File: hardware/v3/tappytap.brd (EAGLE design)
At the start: 36 x 16 mm, 18 parts

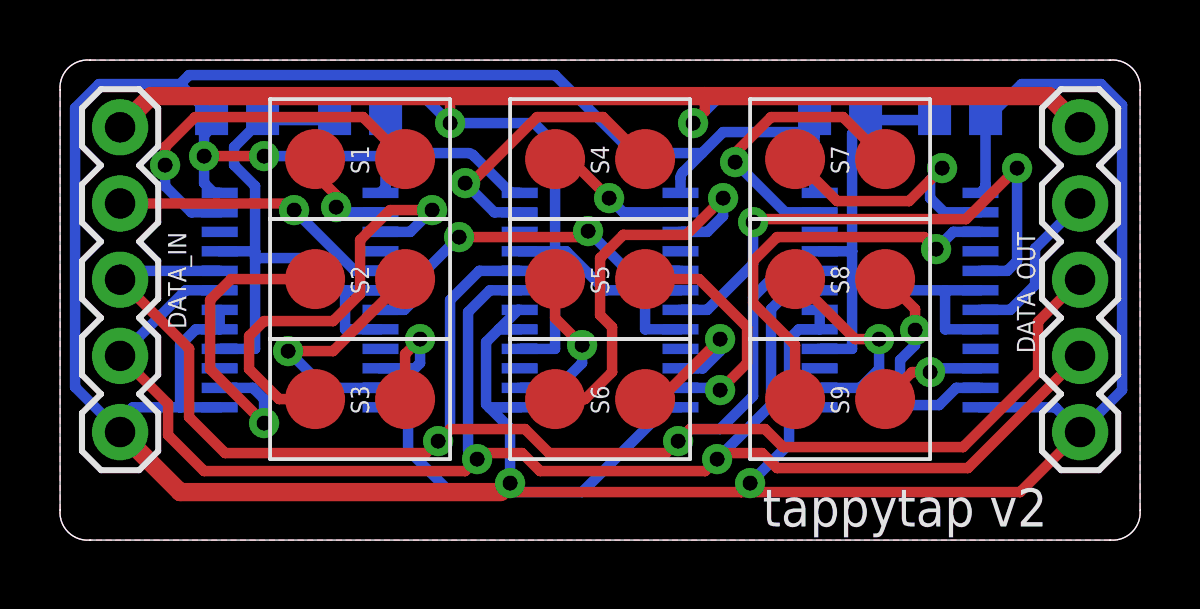
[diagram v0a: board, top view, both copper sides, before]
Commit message: Tappytap v3 design done with gerbers
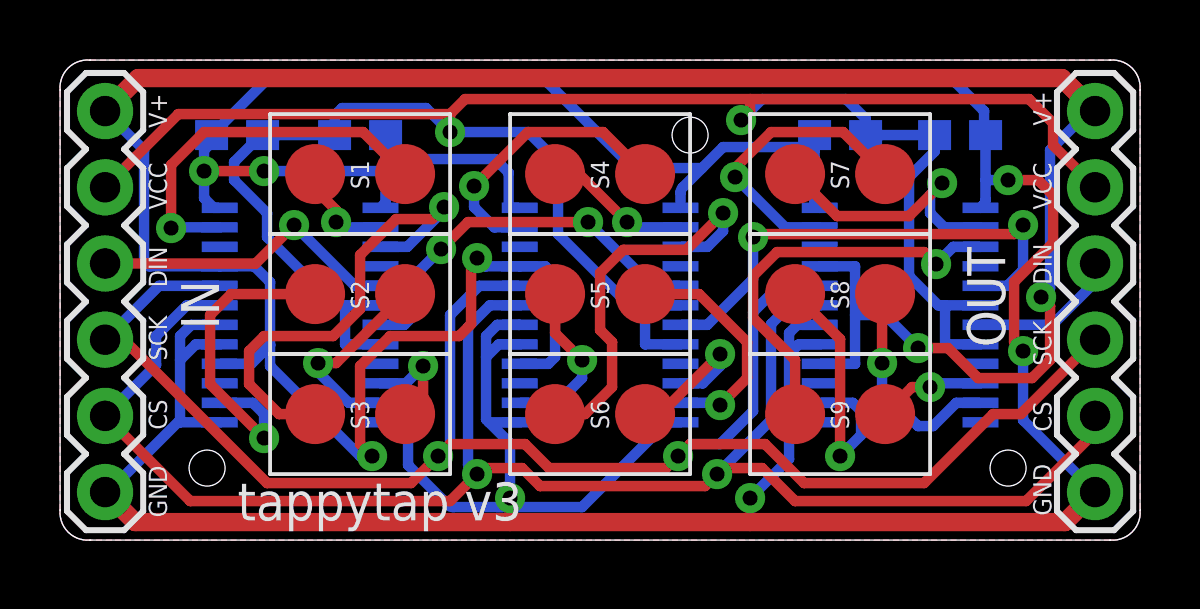
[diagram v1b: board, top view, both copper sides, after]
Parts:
- removed DATA_IN, DATA_OUT: (no value), SparkFun-Connectors:1X05
- added IN, OUT: (no value), SparkFun-Connectors:1X06
- moved C1 0.50 mm to (5.90, 12.5)
- moved C2 0.50 mm to (10.0, 12.5)
- moved C3 0.50 mm to (26.0, 12.5)
- moved C4 0.50 mm to (30.0, 12.5)
- moved HBR1 0.50 mm to (8.00, 6.50)
- moved HBR2 0.50 mm to (18.0, 6.50)
- moved HBR3 0.50 mm to (28.0, 6.50)
- moved S1 0.50 mm to (10.0, 11.2)
- moved S2 0.50 mm to (10.0, 7.20)
- moved S3 0.50 mm to (10.0, 3.20)
- moved S4 0.50 mm to (18.0, 11.2)
- moved S5 0.50 mm to (18.0, 7.20)
- moved S6 0.50 mm to (18.0, 3.20)
- moved S7 0.50 mm to (26.0, 11.2)
- moved S8 0.50 mm to (26.0, 7.20)
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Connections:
- new net V+: HBR1.16, HBR1.21, HBR2.16, HBR2.21, HBR3.16, HBR3.21, IN.6, OUT.6
- net +5V: now also IN.5, OUT.5; no longer DATA_IN.5, DATA_OUT.5, HBR1.16, HBR1.21, HBR2.16, HBR2.21, HBR3.16, HBR3.21
- net GND: now also IN.1, OUT.1; no longer DATA_IN.1, DATA_OUT.1
- net NCV_CS: now also IN.2, OUT.2; no longer DATA_IN.2, DATA_OUT.2
- net SCK: now also IN.3, OUT.3; no longer DATA_IN.3, DATA_OUT.3
- net SI: now also IN.4; no longer DATA_IN.4
- net SO: now also OUT.4; no longer DATA_OUT.4
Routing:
- net V+: track 0.00 -> 93.7 mm, vias 0 -> 4
- net +5V: track 106.8 -> 88.4 mm
- net S8A: track 6.87 -> 9.31 mm
- net NCV_CS: track 55.6 -> 57.7 mm
- net S2B: track 8.48 -> 6.66 mm
- net N$26: track 18.5 -> 16.8 mm
- net S3A: track 14.6 -> 16.0 mm
- net N$24: track 12.0 -> 13.1 mm
- net SI: track 9.61 -> 10.5 mm
- net S3B: track 4.40 -> 3.51 mm
- net GND: track 156.1 -> 156.2 mm, vias 4 -> 6
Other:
- board text added: "CS"
- board text added: "DIN"
- board text added: "GND"
- board text added: "SCK"
- board text added: "V+"
- board text added: "VCC"
- board text added: "tappytap v3"
- board text removed: "tappytap v2"
